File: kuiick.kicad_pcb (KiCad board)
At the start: 2 copper layers, 15 x 19 mm, 22 parts, among them J1 10118193-0001LF, J2 I2C_STANDARDQWIIC, J3 Conn_01x07, J4 Conn_01x07, SW1 SW_SPST, SW2 SW_SPST, U1 MK32L2B_QFN32, U2 W25Q32JVSS

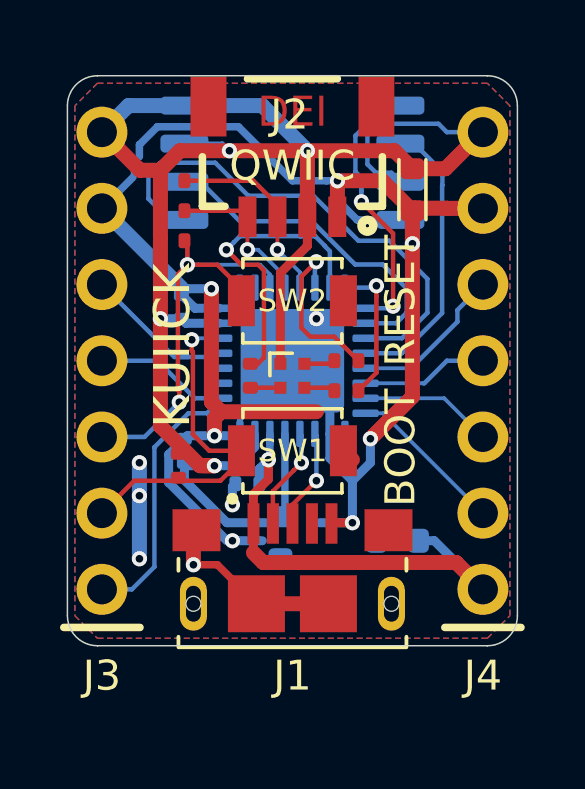
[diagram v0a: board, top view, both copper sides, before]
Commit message: fully routed dip 16
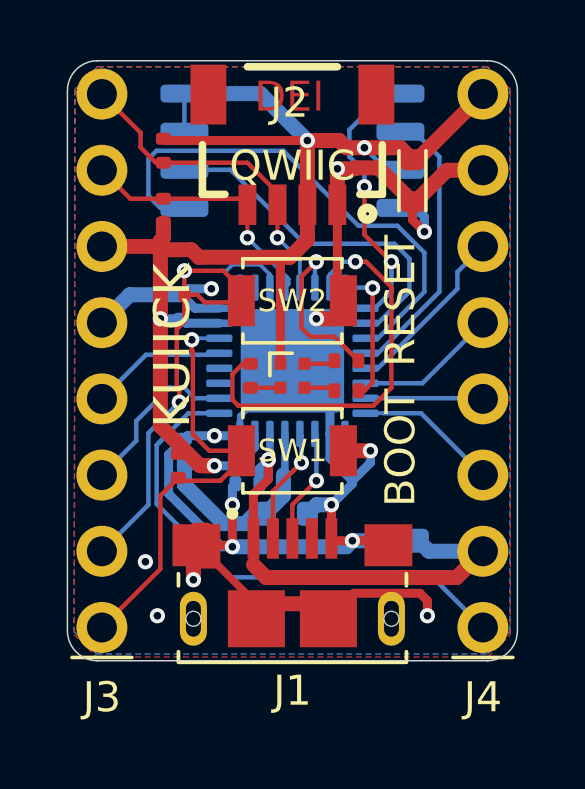
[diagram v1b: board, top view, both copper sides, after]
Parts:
- J3, J4: value Conn_01x07 -> Conn_01x08; footprint footprint:PinHeader_1x07_P100mil_Vertical -> footprint:PinHeader_1x08_P100mil_Vertical
- moved R7 1.80 mm to (146.0, 97.8)
- moved J3 1.27 mm to (143.7, 108.9)
- moved J4 1.27 mm to (156.3, 108.9)
- moved R5 1.04 mm to (145.7, 93.0), turned to 90 degrees
- moved C1 0.82 mm to (149.8, 105.1), turned to 0 degrees
- moved J1 0.50 mm to (150.0, 108.6)
- moved J2 0.40 mm to (150.0, 94.8)
- moved U2 0.40 mm to (150.0, 93.0)
- moved R4 0.30 mm to (145.7, 95.0), turned to -90 degrees
- moved C8 0.30 mm to (154.0, 94.0)
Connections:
- J3 pad 1: /AN -> /NMI#
- J3 pad 2: /NMI# -> /RST#
- J3 pad 3: /RST# -> /SWC
- J3 pad 4: /SWC -> /SWD
- J3 pad 5: /SWD -> GND
- J3 pad 6: GND -> /3V3
- J3 pad 7: /3V3 -> /SCL
- J4 pad 1: /+5V -> /AN
- J4 pad 2: /FX7 -> /+5V
- J4 pad 3: /FX6 -> /FX7
- J4 pad 4: /FX5 -> /FX6
- J4 pad 5: /FX4 -> /FX5
- J4 pad 6: GND -> /FX4
- J4 pad 7: /3V3 -> GND
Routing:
- net GND: track 80.8 -> 66.5 mm, vias 13 -> 14
- net /AN: track 8.68 -> 17.6 mm
- net /3V3: track 61.3 -> 56.6 mm
- net /SDA: track 6.51 -> 11.0 mm
- net /RST#: track 14.9 -> 19.4 mm
- net /SCL: track 5.28 -> 8.89 mm
- net /G: track 10.4 -> 13.6 mm
- net /NMI#: track 12.2 -> 15.0 mm
- net /SWC: track 4.43 -> 5.65 mm
- net /SWD: track 5.21 -> 4.32 mm
- net /MOSI: track 16.9 -> 17.7 mm
- net /FX4: track 5.30 -> 5.92 mm
- net /FX6: track 4.45 -> 3.92 mm
- net /FX7: track 5.29 -> 4.77 mm
- net /FX5: track 4.22 -> 4.75 mm
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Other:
- board size 15 x 19 mm -> 15 x 20 mm
